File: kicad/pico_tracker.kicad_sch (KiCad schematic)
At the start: 28 parts, among them J1 MIDI_OUT, J10 DclassAMP, J11 MASTER_VOLUME, J2 MIDI_IN, J3 MIDI_IN_A_B_VCC, J4 MIDI_IN_A_B_DATA, J5 MIDI_OUT_A_B_VCC, J6 MIDI_OUT_A_B_DATA, J7 DISPLAY, J8 SDCARD, J9 KILL_SWITCH, SW1 LEFT, SW2 DOWN, SW3 RIGHT, SW4 UP, SW5 RT, SW6 B, SW7 A, SW8 LT, SW9 PLAY, U1 Pico, U2 6N138, U3 PCM5102_Module

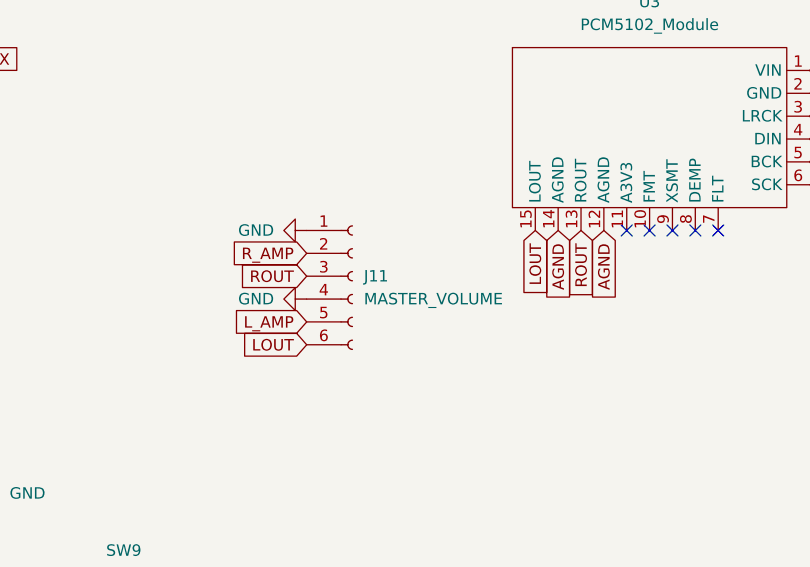
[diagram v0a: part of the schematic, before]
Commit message: Add files via upload
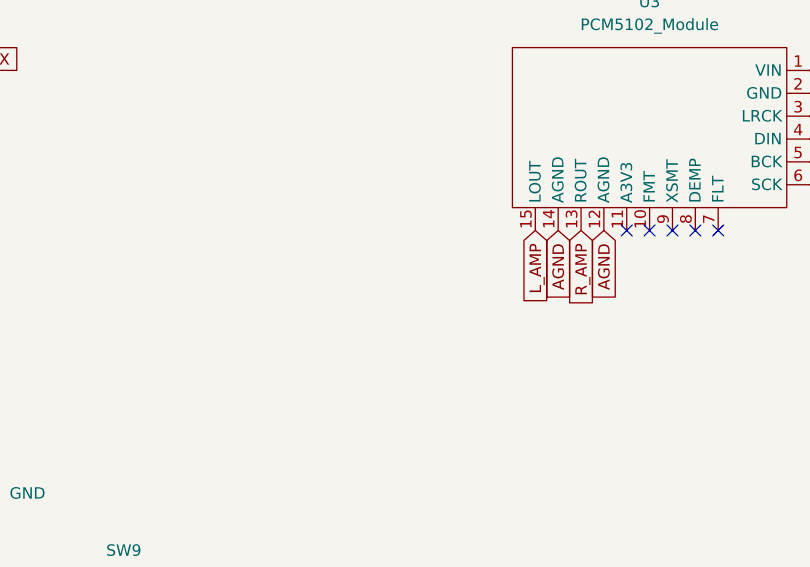
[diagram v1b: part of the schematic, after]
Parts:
- removed J11: MASTER_VOLUME, Connector_PinHeader_2.54mm:PinHeader_2x03_P2.54mm_Vertical_SMD, symbol Connector:Conn_01x06_Female
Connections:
- net LOUT is gone; now on net L_AMP: U3.15 (LOUT)
- net ROUT is gone; now on net R_AMP: U3.13 (ROUT)
